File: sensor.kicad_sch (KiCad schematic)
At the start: 26 parts, among them J14 RadEye1, U44 SN74AVC8T245PW, U45 AD5112, U46 INA849

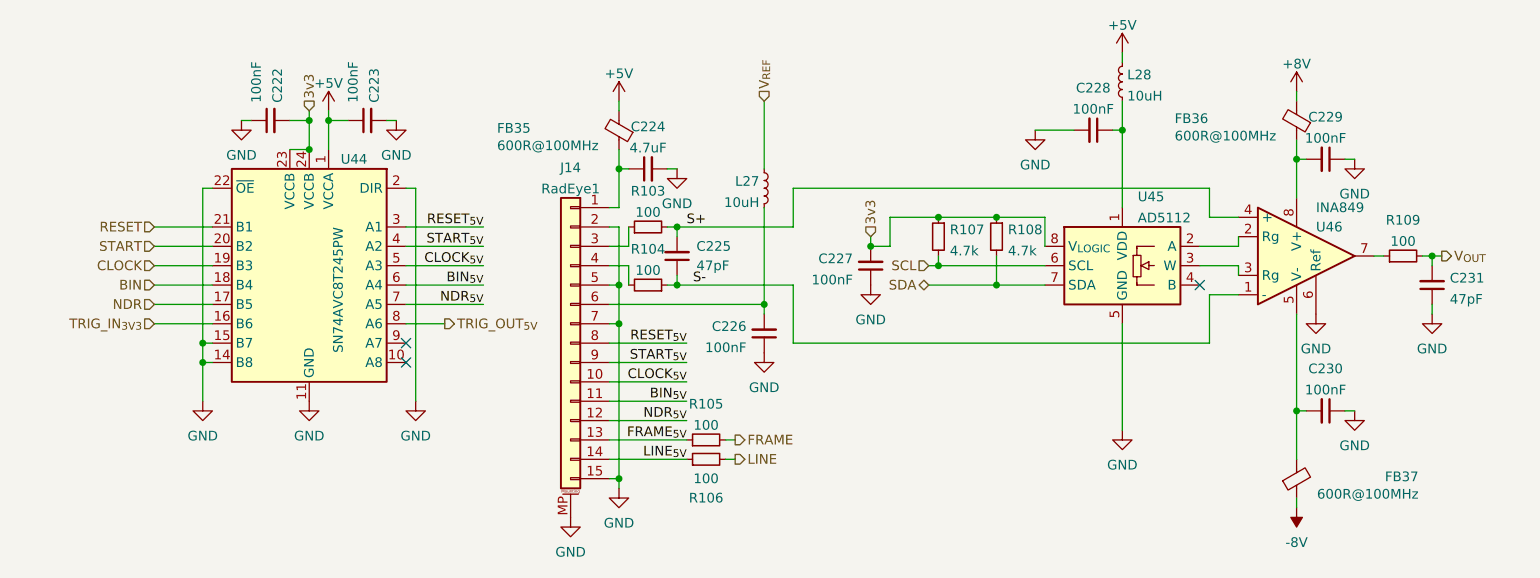
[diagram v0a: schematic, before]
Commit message: Use two instead of four 3.8V voltage references
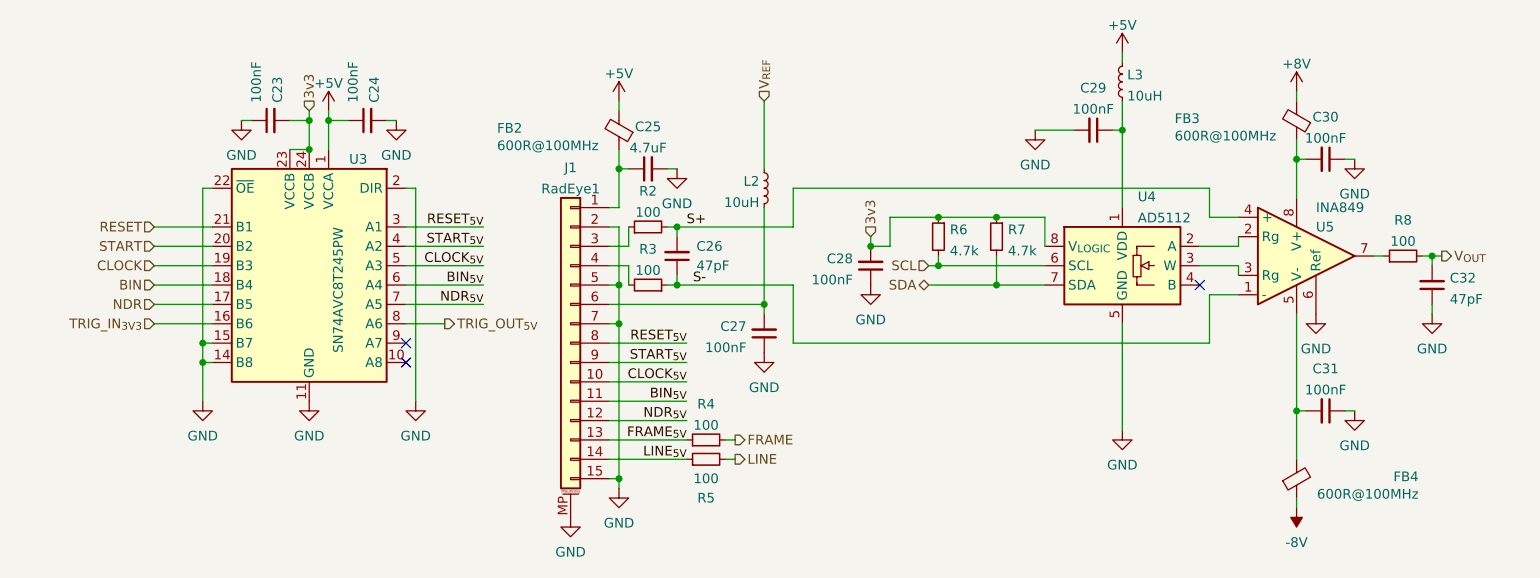
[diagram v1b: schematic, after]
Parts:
- renumbered C222 to C23, C223 to C24, C224 to C25, C225 to C26, C226 to C27, C227 to C28, C228 to C29, C229 to C30, C230 to C31, C231 to C32, FB35 to FB2, FB36 to FB3, FB37 to FB4, J14 to J1, L27 to L2, L28 to L3, R103 to R2, R104 to R3, R105 to R4, R106 to R5, R107 to R6, R108 to R7, R109 to R8, U44 to U3, U45 to U4, U46 to U5

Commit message: Add sensor board power planes
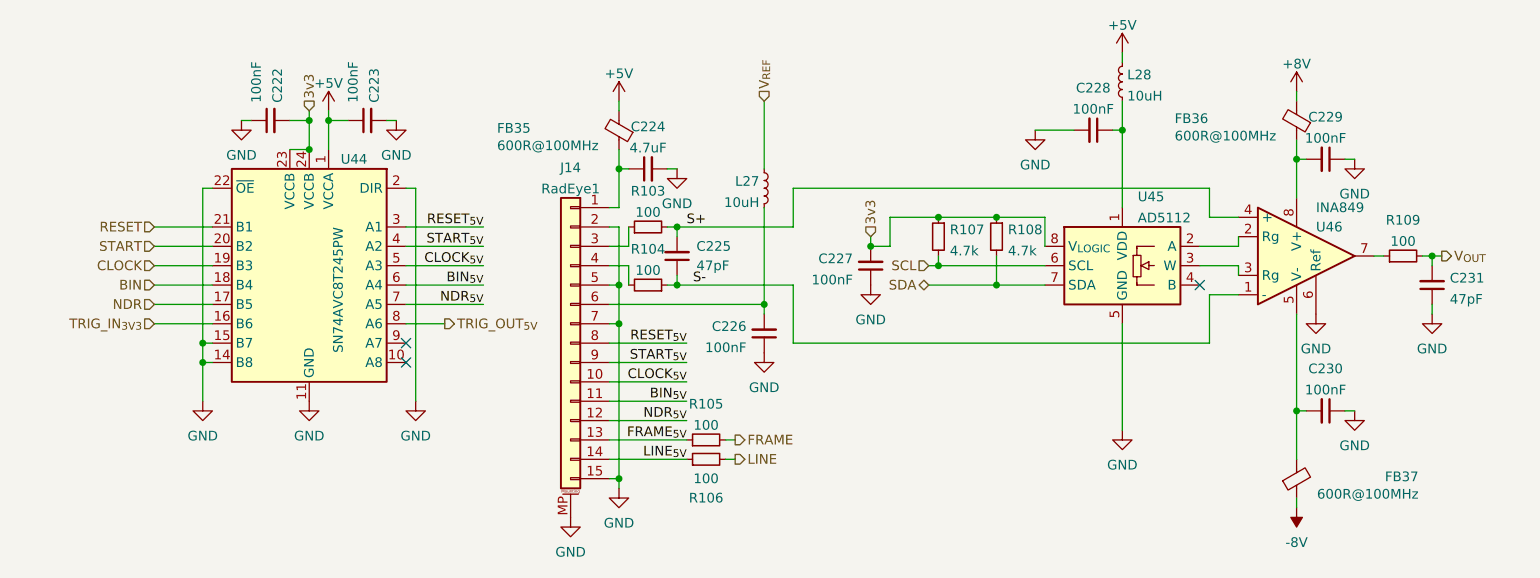
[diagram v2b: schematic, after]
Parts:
- renumbered C23 to C222, C24 to C223, C25 to C224, C26 to C225, C27 to C226, C28 to C227, C29 to C228, C30 to C229, C31 to C230, C32 to C231, FB2 to FB35, FB3 to FB36, FB4 to FB37, J1 to J14, L2 to L27, L3 to L28, R2 to R103, R3 to R104, R4 to R105, R5 to R106, R6 to R107, R7 to R108, R8 to R109, U3 to U44, U4 to U45, U5 to U46
